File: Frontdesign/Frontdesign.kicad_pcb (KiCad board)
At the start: 2 copper layers, 147.3 x 147.3 mm, 0 parts

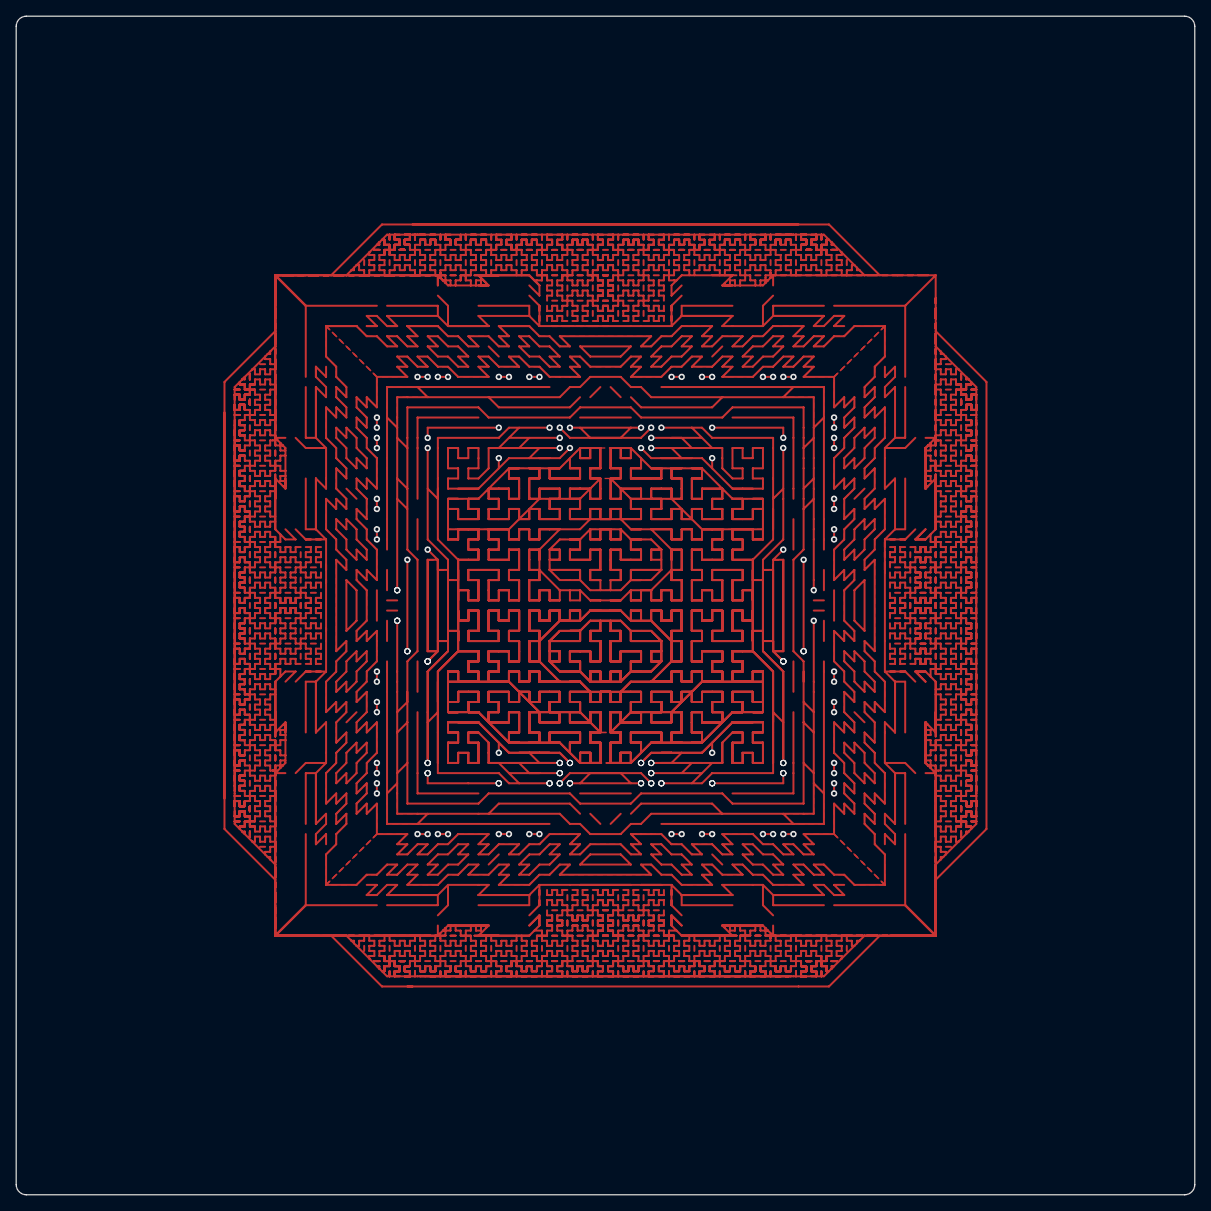
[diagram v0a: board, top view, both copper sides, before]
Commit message: changes in frontdesign
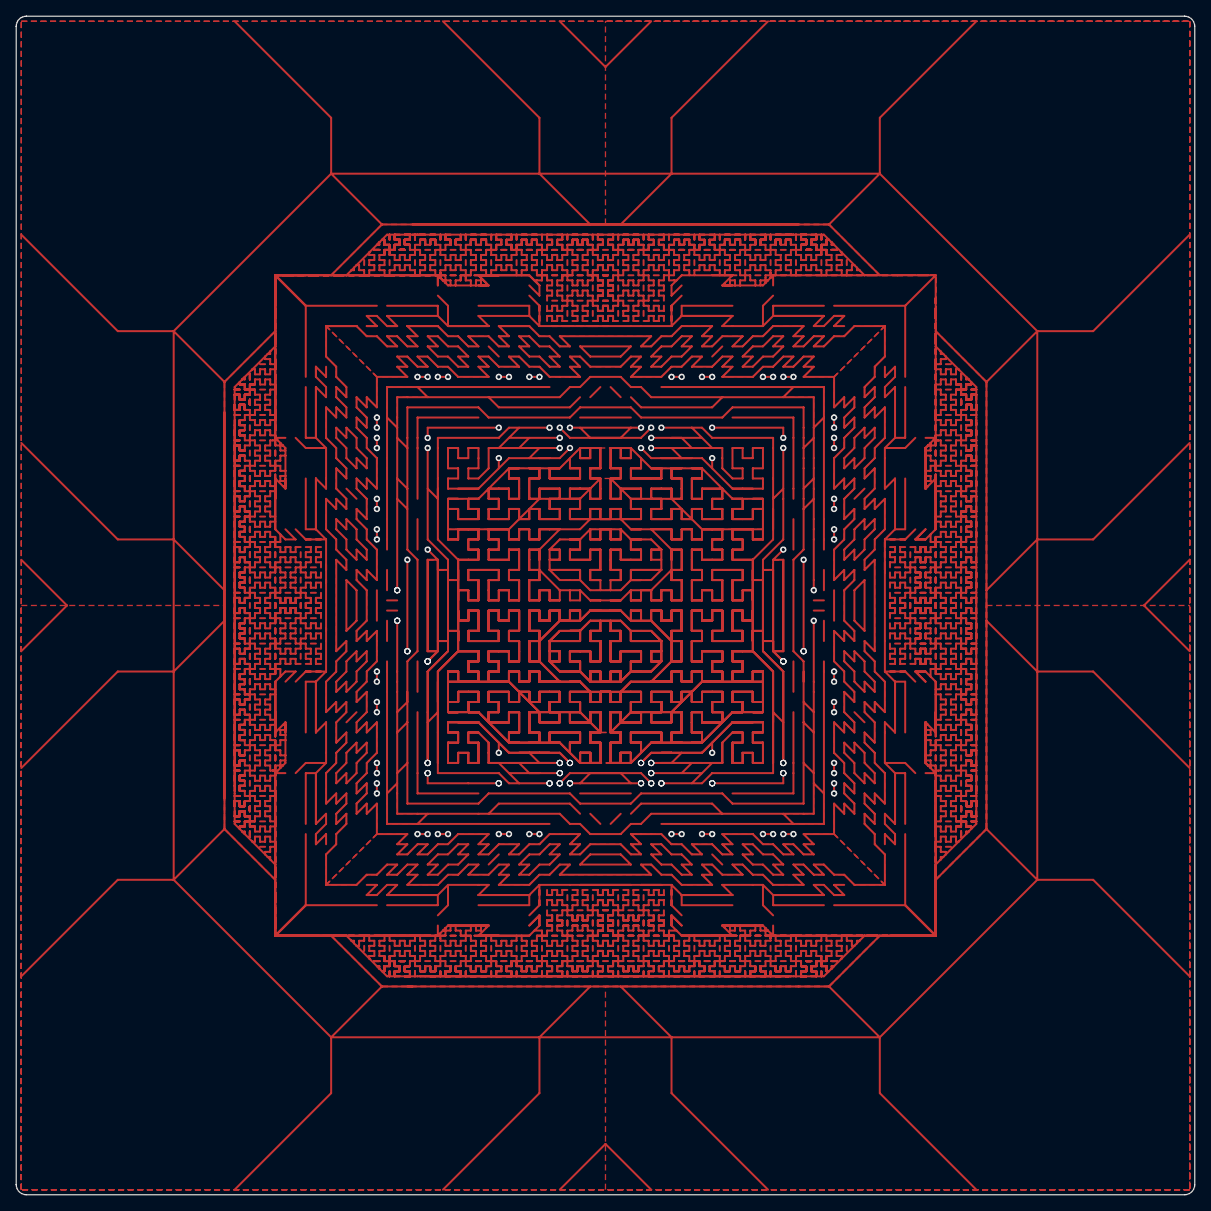
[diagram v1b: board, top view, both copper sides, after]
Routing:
- net (no net): track 12814.4 -> 13793.1 mm
